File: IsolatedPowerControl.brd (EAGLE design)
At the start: 160 x 100 mm, 39 parts, among them IC1 LM358, Q1 FDN360P, U1 MCP23008-E/SO, U2 MCP4716A0T-E/CH

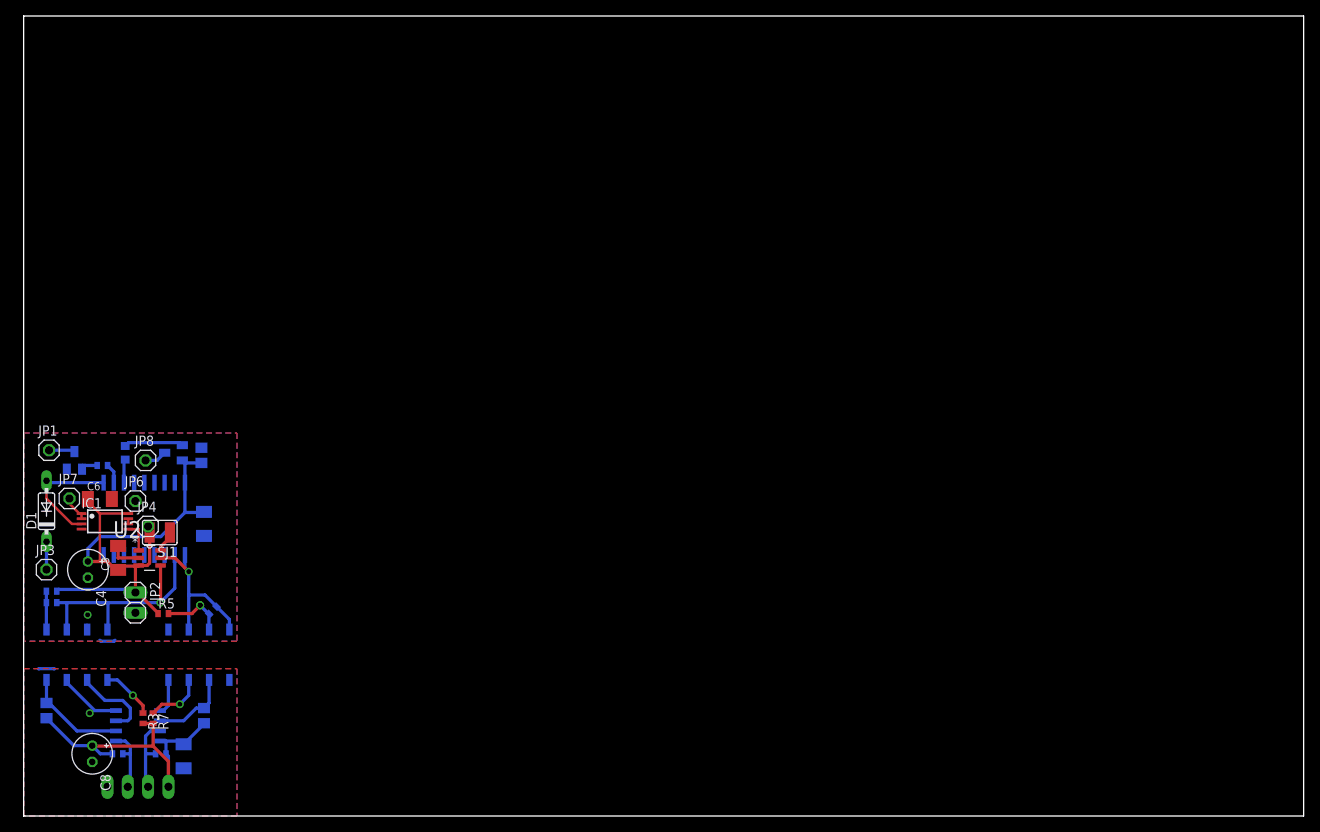
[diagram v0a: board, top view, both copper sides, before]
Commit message: First layout complete and checked
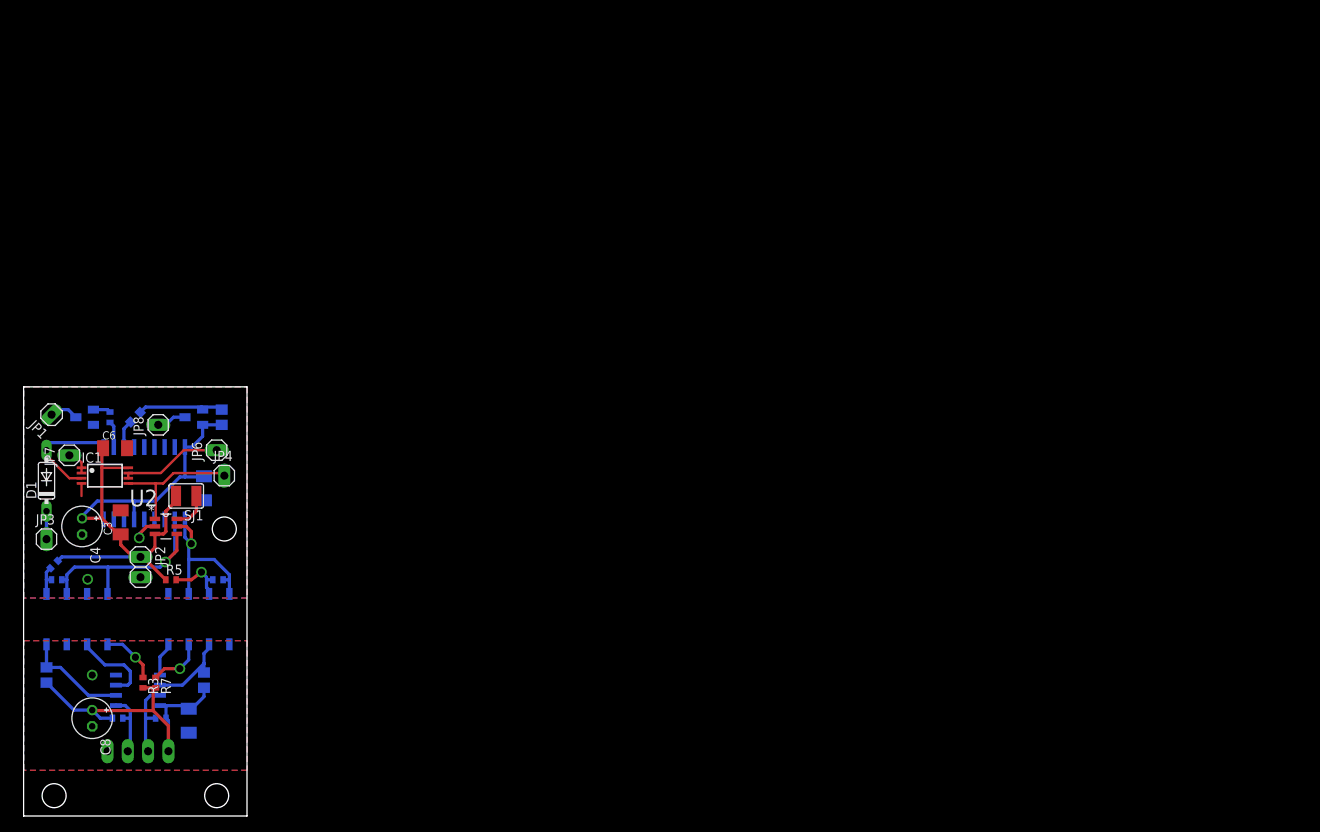
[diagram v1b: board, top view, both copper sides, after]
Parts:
- JP1, JP3, JP4, JP6, JP7, JP8: device pinhead:1X01 -> pinhead:1X01-LARGEPAD
- moved JP6 12.0 mm to (24.1, 45.7), turned to 90 degrees
- moved JP4 11.4 mm to (25.1, 42.5)
- moved C6 6.63 mm to (11.4, 46.0)
- moved R11 6.11 mm to (10.8, 49.8), turned to 90 degrees
- moved IC1 5.72 mm to (10.2, 42.5)
- moved SJ1 5.64 mm to (20.3, 40.0)
- moved T3 5.54 mm to (7.62, 49.8), turned to 270 degrees
- moved C4 5.45 mm to (7.30, 36.2)
- moved JP7 5.40 mm to (5.71, 45.1), turned to 90 degrees
- moved R14 5.40 mm to (24.8, 49.8)
- moved Q1 5.12 mm to (21.3, 49.8)
- moved JP8 4.72 mm to (16.8, 48.9), turned to 90 degrees
- moved R12 4.62 mm to (14.0, 49.8), turned to 315 degrees
- moved C7 4.49 mm to (20.6, 11.9)
- moved JP2 4.49 mm to (14.6, 31.1)
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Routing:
- net VPOWER: track 4.07 -> 17.1 mm
- net VPOWER_BUFFERED: track 0.65 -> 12.9 mm
- net GND: track 9.92 -> 0.34 mm
- net V+: track 69.0 -> 78.2 mm
- net N$12: track 7.44 -> 11.0 mm
- net V-: track 6.93 -> 4.90 mm, vias 1 -> 2
- net N$11: track 2.87 -> 4.74 mm
- net SDA: track 31.1 -> 29.3 mm
- net SCL: track 21.3 -> 22.4 mm
- net N$13: track 2.79 -> 3.74 mm
- net RY-SCL: track 9.94 -> 10.8 mm
- net RELAYONOFF: track 2.47 -> 3.28 mm
- net N$2: track 4.79 -> 4.07 mm
- net DIRECTONOFF: track 15.3 -> 14.7 mm
- net N$5: track 7.95 -> 7.37 mm, vias 2 -> 1
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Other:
- board size 160 x 100 mm -> 27.9 x 53.6 mm
